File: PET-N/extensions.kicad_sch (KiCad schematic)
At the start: 78 parts, among them SW1 KP "=", SW10 KP "0", SW11 R SHIFT, SW12 ">", SW14 "]", SW15 "@", SW16 L SHIFT, SW17 KP "+", SW18 KP "2", SW2 KP ".", SW20 "?", SW21 ",", SW22 "N", SW23 "V", SW24 "X", SW25 KP "3", SW26 KP "1", SW27 RETURN, SW28 ";", SW29 "M", SW3 NC ($10), SW30 "B", SW31 "C", SW32 "Z", SW320 S LOCK, SW33 KP "*", SW34 KP "5", SW36 ":", SW37 "K", SW38 "H", SW39 "F", SW4 STOP, SW40 "S", SW41 KP "6", SW42 KP "4", SW44 "L", SW45 "J", SW46 "G", SW47 "D", SW48 "A", SW49 KP "/", SW5 "<", SW50 KP "8", SW52 "P", SW53 "I", SW54 "Y", SW55 "R", SW56 "W", SW57 KP "9", SW58 KP "7", SW59 U ARROW, SW6 SPACE, SW60 "O", SW61 "U", SW62 "T", SW63 "E", SW64 "Q", SW65 INS/DEL, SW66 UP/DOWN, SW67 NC ($0A), SW68 ")", SW69 "\", SW7 "[", SW70 "'", SW71 "$", SW72 QUOTE, SW73 LEFT/RIGHT, SW74 CLR/HOME, SW75 B ARROW, SW76 "(", SW77 "&", SW78 "%", SW79 "#", SW8 OFF/RVS, SW80 "!", SW9 KP "-", U1 74LS145

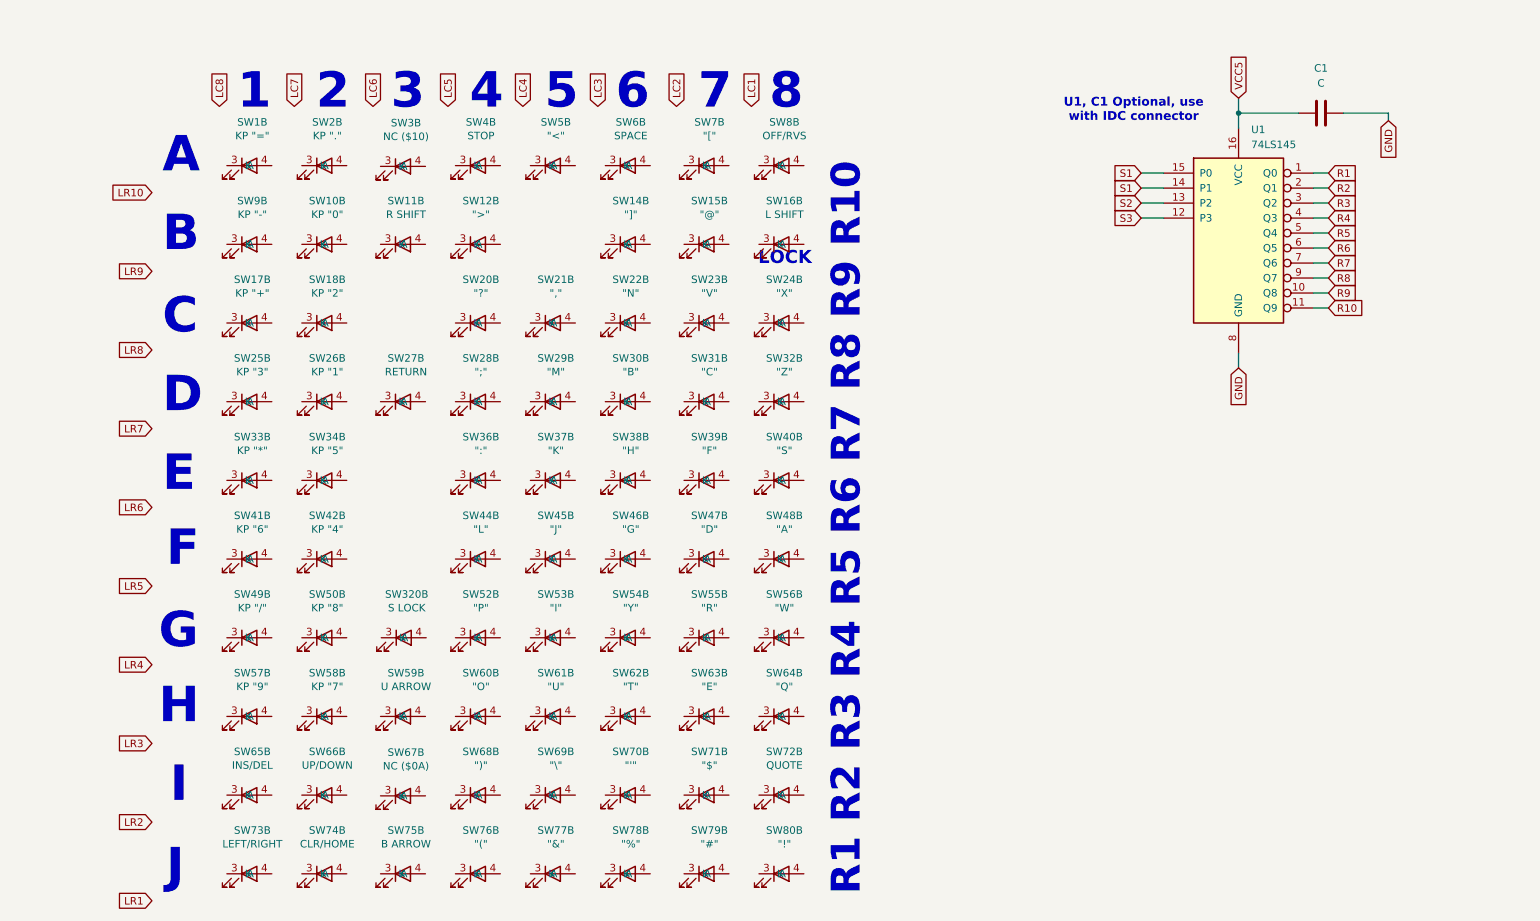
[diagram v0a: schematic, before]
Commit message: work on R3 of keyboard pcb
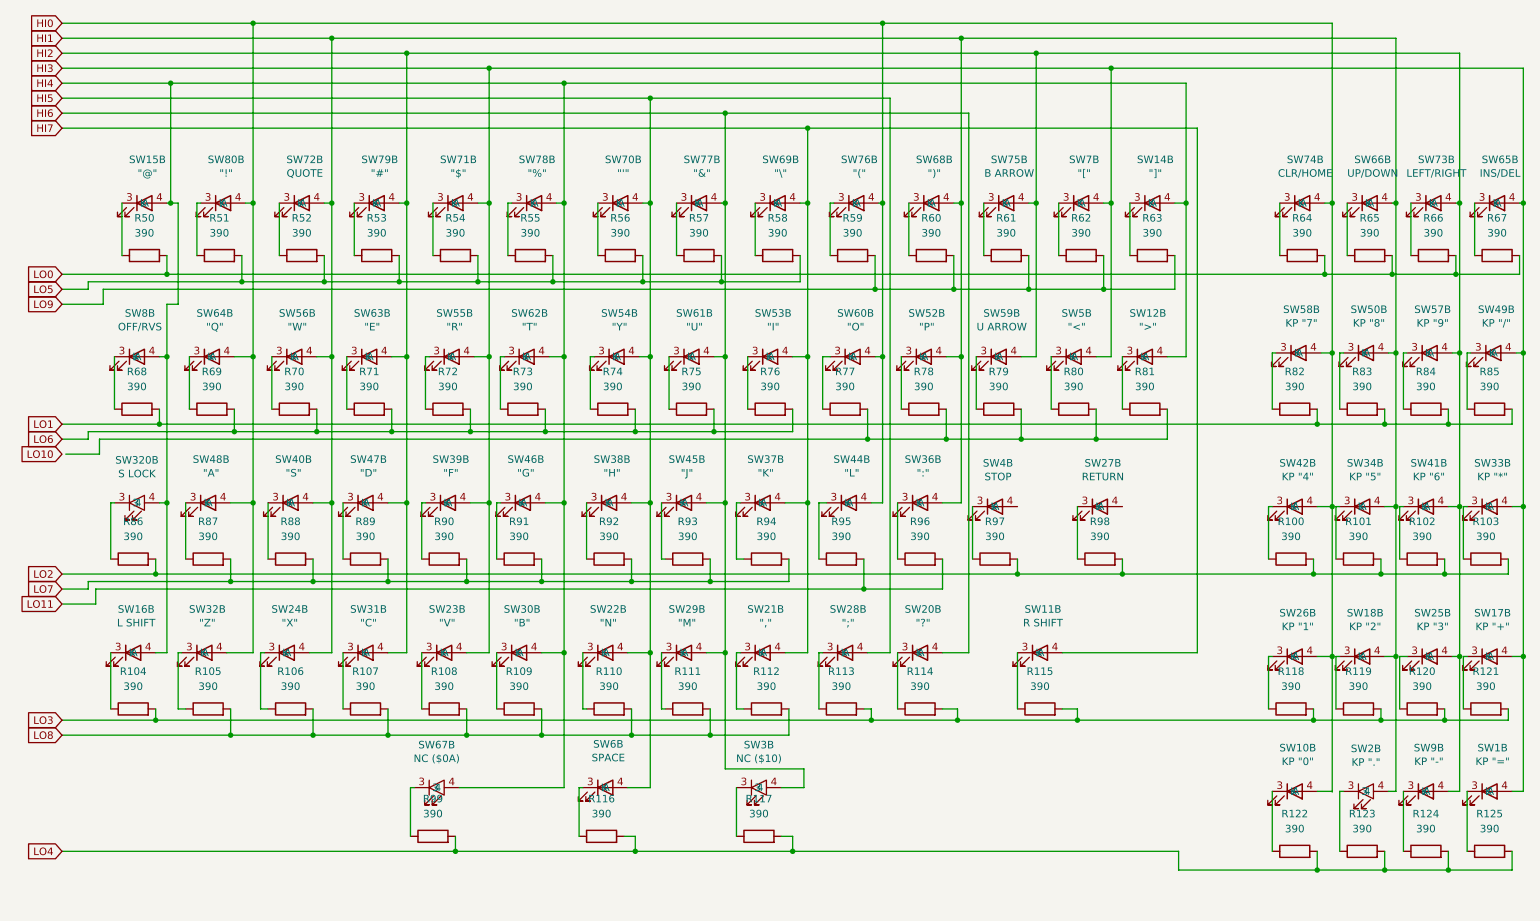
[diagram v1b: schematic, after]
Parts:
- removed C1: C, Capacitor_THT:C_Disc_D4.3mm_W1.9mm_P5.00mm, symbol Device:C
- removed U1: 74LS145, Package_DIP:DIP-16_W7.62mm, symbol 74xx:74LS145
- added R100, R101, R102, R103, R104, R105, R106, R107, R108, R109, R110, R111, R112, R113, R114, R115, R116, R117, R118, R119, R120, R121, R122, R123, R124, R125, R50, R51, R52, R53, R54, R55, R56, R57, R58, R59, R60, R61, R62, R63, R64, R65, R66, R67, R68, R69, R70, R71, R72, R73, R74, R75, R76, R77, R78, R79, R80, R81, R82, R83, R84, R85, R86, R87, R88, R89, R90, R91, R92, R93, R94, R95, R96, R97, R98, R99: 390, Resistor_SMD:R_0805_2012Metric, symbol Device:R
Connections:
- net at SW11.3 (K): now also R115.1
- net HI7: now reaches SW11.4 (A)
- net HI7: now also SW21.4 (A), SW37.4 (A), SW53.4 (A), SW69.4 (A)
- net at SW70.3 (K): now also R56.1
- net HI5: now reaches SW70.4 (A)
- net HI5: now also SW22.4 (A), SW28.4 (A), SW38.4 (A), SW54.4 (A), SW6.4 (A)
- net at SW34.3 (K): now also R101.1
- net HI1: now reaches SW34.4 (A)
- net HI1: now also SW18.4 (A), SW2.4, SW24.4 (A), SW36.4 (A), SW40.4 (A), SW50.4 (A), SW52.4 (A), SW56.4 (A), SW66.4 (A), SW68.4 (A), SW72.4 (A)
- net at SW65.3 (K): now also R67.1
- net HI3: now reaches SW65.4 (A)
- net HI3: now also SW1.4 (A), SW17.4 (A), SW23.4 (A), SW33.4 (A), SW39.4 (A), SW49.4 (A), SW5.4 (A), SW55.4 (A), SW7.4 (A), SW71.4 (A)
- net at SW18.3 (K): now also R119.1
- net at SW72.3 (K): now also R52.1
- net at SW39.3 (K): now also R90.1
- net at SW1.3 (K): now also R125.1
- net at SW47.3 (K): now also R89.1
- net HI2: now reaches SW47.4 (A)
- net HI2: now also SW25.4 (A), SW31.4 (A), SW41.4 (A), SW57.4 (A), SW59.4 (A), SW63.4 (A), SW73.4 (A), SW75.4 (A), SW79.4 (A), SW9.4 (A)
- net at SW5.3 (K): now also R80.1
- net at SW49.3 (K): now also R85.1
- net at SW78.3 (K): now also R55.1
- net HI4: now reaches SW78.4 (A)
- net HI4: now also SW12.4 (A), SW14.4 (A), SW15.4 (A), SW16.4 (A), SW30.4 (A), SW320.4, SW46.4 (A), SW62.4 (A), SW67.4, SW8.4 (A)
- net at SW32.3 (K): now also R105.1
- net HI0: now reaches SW32.4 (A)
- net HI0: now also SW26.4 (A), SW42.4 (A), SW44.4 (A), SW48.4 (A), SW58.4 (A), SW60.4 (A), SW64.4 (A), SW74.4 (A), SW76.4 (A), SW80.4 (A)
- net at SW64.3 (K): now also R69.1
- net at SW48.3 (K): now also R87.1
- net at SW15.3 (K): now also R50.1
- net at SW2.3: now also R123.1
- net at SW55.3 (K): now also R72.1
- net at SW8.3 (K): now also R68.1
- net at SW4.3 (K): now also R97.1
- net at SW37.3 (K): now also R94.1
- net at SW71.3 (K): now also R54.1
- net at SW3.3: now also R117.1
- net HI6: now reaches SW3.4
- net HI6: now also SW20.4 (A), SW29.4 (A), SW45.4 (A), SW61.4 (A), SW77.4 (A)
- net at SW56.3 (K): now also R70.1
- net at SW75.3 (K): now also R61.1
- net at SW6.3 (K): now also R116.1
- net at SW69.3 (K): now also R58.1
- net at SW24.3 (K): now also R106.1
- net at SW16.3 (K): now also R104.1
- net at SW320.3: now also R86.1
- net at SW36.3 (K): now also R96.1
- net at SW62.3 (K): now also R73.1
- net at SW20.3 (K): now also R114.1
- net at SW17.3 (K): now also R121.1
- net at SW45.3 (K): now also R93.1
- net at SW66.3 (K): now also R65.1
- net at SW50.3 (K): now also R83.1
- net at SW7.3 (K): now also R62.1
- net at SW31.3 (K): now also R107.1
- net at SW52.3 (K): now also R78.1
- net at SW46.3 (K): now also R91.1
- net at SW67.3: now also R99.1
- net at SW59.3 (K): now also R79.1
- net at SW14.3 (K): now also R63.1
- net at SW73.3 (K): now also R66.1
- net at SW33.3 (K): now also R103.1
- net at SW25.3 (K): now also R120.1
- net at SW60.3 (K): now also R77.1
- net at SW10.3 (K): now also R122.1
- net at SW27.3 (K): now also R98.1
- net at SW38.3 (K): now also R92.1
- net at SW29.3 (K): now also R111.1
- net at SW9.3 (K): now also R124.1
- net at SW26.3 (K): now also R118.1
- net at SW63.3 (K): now also R71.1
- net at SW68.3 (K): now also R60.1
- net at SW21.3 (K): now also R112.1
- net at SW22.3 (K): now also R110.1
- net at SW53.3 (K): now also R76.1
- net at SW41.3 (K): now also R102.1
- net at SW58.3 (K): now also R82.1
- net at SW76.3 (K): now also R59.1
- net at SW40.3 (K): now also R88.1
- net at SW54.3 (K): now also R74.1
- net at SW61.3 (K): now also R75.1
- net at SW28.3 (K): now also R113.1
- net at SW80.3 (K): now also R51.1
- net at SW79.3 (K): now also R53.1
- net at SW77.3 (K): now also R57.1
- net at SW57.3 (K): now also R84.1
- net at SW30.3 (K): now also R109.1
- net at SW12.3 (K): now also R81.1
- net at SW42.3 (K): now also R100.1
- net at SW23.3 (K): now also R108.1
- net at SW44.3 (K): now also R95.1
- net at SW74.3 (K): now also R64.1
- new net: R77.2, R78.2, R79.2, R80.2, R81.2
- new net LO0: R50.2, R64.2, R65.2, R66.2, R67.2
- new net LO1: R68.2, R82.2, R83.2, R84.2, R85.2
- new net LO11: R95.2, R96.2
- new net LO2: R100.2, R101.2, R102.2, R103.2, R86.2, R97.2, R98.2
- new net LO3: R104.2, R113.2, R114.2, R115.2, R118.2, R119.2, R120.2, R121.2
- new net LO4: R116.2, R117.2, R122.2, R123.2, R124.2, R125.2, R99.2
- new net LO5: R51.2, R52.2, R53.2, R54.2, R55.2, R56.2, R57.2, R58.2
- new net LO6: R69.2, R70.2, R71.2, R72.2, R73.2, R74.2, R75.2, R76.2
- new net LO7: R87.2, R88.2, R89.2, R90.2, R91.2, R92.2, R93.2, R94.2
- new net LO8: R105.2, R106.2, R107.2, R108.2, R109.2, R110.2, R111.2, R112.2
- new net LO9: R59.2, R60.2, R61.2, R62.2, R63.2
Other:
- note removed: "1"
- note removed: "2"
- note removed: "3"
- note removed: "4"
- note removed: "5"
- note removed: "6"
- note removed: "7"
- note removed: "8"
- note removed: "A"
- note removed: "B"
- note removed: "C"
- note removed: "D"
- note removed: "E"
- note removed: "F"
- note removed: "G"
- note removed: "H"
- note removed: "I"
- note removed: "J"
- note removed: "LOCK"
- note removed: "R1 R2 R3 R4 R5 R6 R7 R8 R9 R10"
- note removed: "U1, C1 Optional, use with IDC connector"
- moved on the sheet: SW10B, SW11B, SW12B, SW14B, SW15B, SW16B, SW17B, SW18B, SW1B, SW20B, SW21B, SW22B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
